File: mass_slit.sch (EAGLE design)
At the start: 31 parts, among them IC1 PIC18F1220P

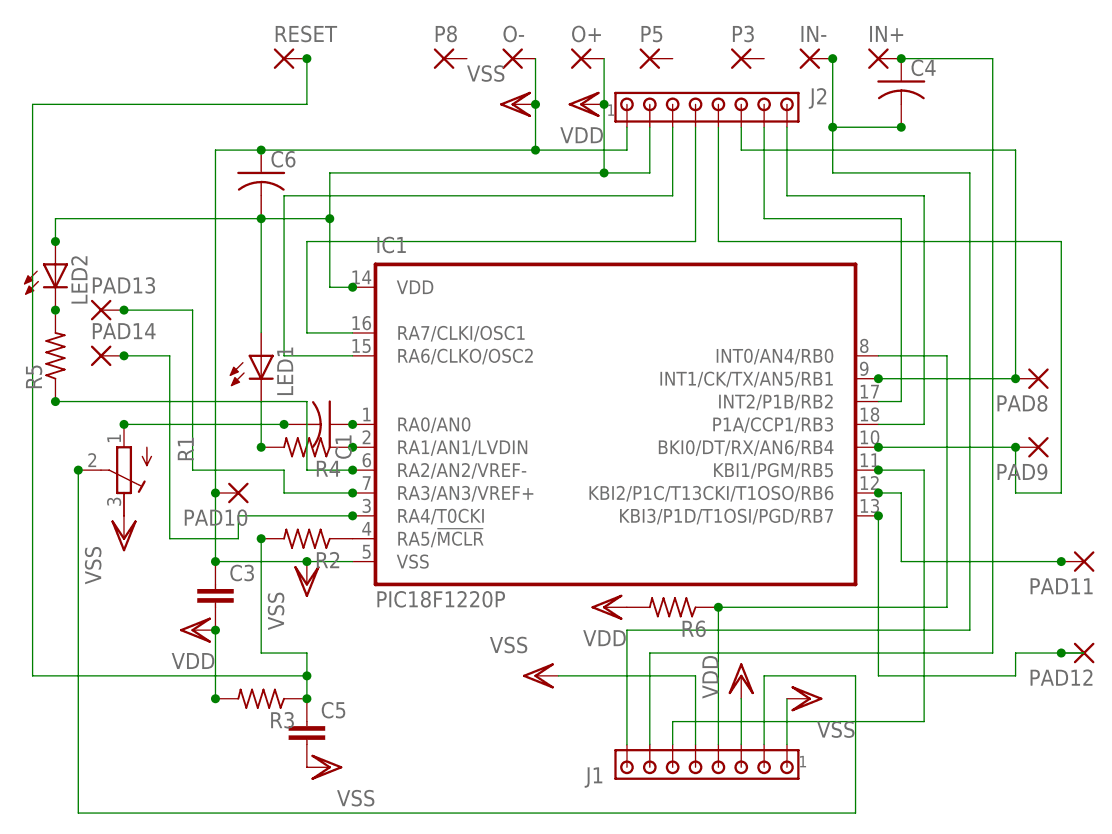
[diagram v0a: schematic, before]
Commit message: up
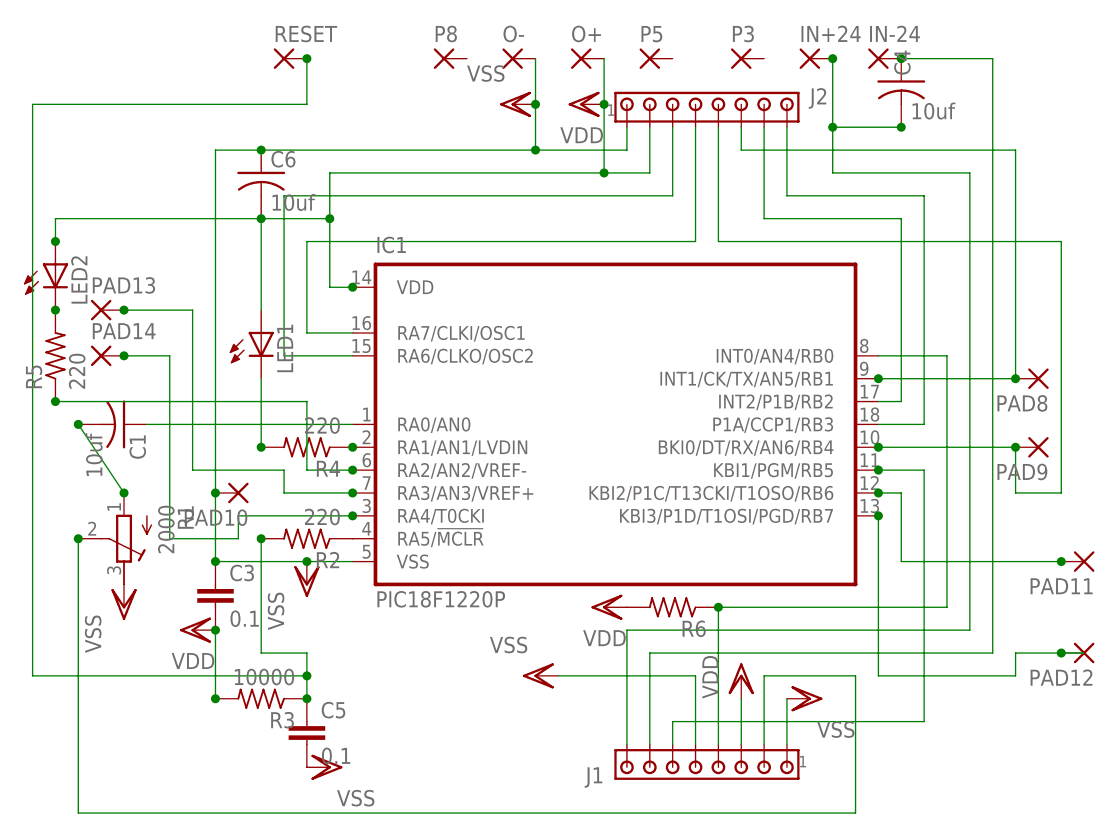
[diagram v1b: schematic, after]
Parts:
- C1, C4, C6: value (none) -> 10uf
- C3, C5: value (none) -> 0.1
- R1: value (none) -> 2000
- R2, R4, R5: value (none) -> 220
- R3: value (none) -> 10000
- renumbered IN+ to IN-24, IN- to IN+24
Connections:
- net N$5 renamed -24
- net N$6 renamed +24
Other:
- moved on the sheet: C1, LED1, R1
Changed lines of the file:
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@@
 <?xml version="1.0" encoding="utf-8"?>
 <!DOCTYPE eagle SYSTEM "eagle.dtd">
-<eagle version="9.2.2">
+<eagle version="9.4.1">
 <drawing>
 <settings>
@@
 <part name="P5" library="wirepad" deviceset="1,6/0,9" device=""/>
 <part name="P3" library="wirepad" deviceset="1,6/0,9" device=""/>
-<part name="IN-" library="wirepad" deviceset="1,6/0,9" device=""/>
-<part name="IN+" library="wirepad" deviceset="1,6/0,9" device=""/>
+<part name="IN+24" library="wirepad" deviceset="1,6/0,9" device=""/>
+<part name="IN-24" library="wirepad" deviceset="1,6/0,9" device=""/>
 <part name="VSS1" library="supply1" deviceset="VSS" device=""/>
-<part name="C1" library="resistor" deviceset="C-US" device="025-040X050"/>
-<part name="C3" library="capacitor-wima" deviceset="C" device="5/2.5"/>
-<part name="C4" library="resistor" deviceset="C-US" device="025-040X050"/>
-<part name="C5" library="capacitor-wima" deviceset="C" device="5/2.5"/>
-<part name="C6" library="resistor" deviceset="C-US" device="025-040X050"/>
+<part name="C1" library="resistor" deviceset="C-US" device="025-040X050" value="10uf"/>
+<part name="C3" library="capacitor-wima" deviceset="C" device="5/2.5" value="0.1"/>
+<part name="C4" library="resistor" deviceset="C-US" device="025-040X050" value="10uf"/>
+<part name="C5" library="capacitor-wima" deviceset="C" device="5/2.5" value="0.1"/>
+<part name="C6" library="resistor" deviceset="C-US" device="025-040X050" value="10uf"/>
 <part name="J1" library="con-amp" deviceset="MTA08-100" device=""/>
-<part name="R1" library="resistor" deviceset="R-TRIMM" device="3339P"/>
-<part name="R2" library="resistor" deviceset="R-US_" device="0204/2V"/>
-<part name="R3" library="resistor" deviceset="R-US_" device="0204/2V"/>
-<part name="R4" library="resistor" deviceset="R-US_" device="0204/2V"/>
+<part name="R1" library="resistor" deviceset="R-TRIMM" device="3339P" value="2000"/>
+<part name="R2" library="resistor" deviceset="R-US_" device="0204/2V" value="220"/>
+<part name="R3" library="resistor" deviceset="R-US_" device="0204/2V" value="10000"/>
+<part name="R4" library="resistor" deviceset="R-US_" device="0204/2V" value="220"/>
 <part name="VSS4" library="supply1" deviceset="VSS" device=""/>
 <part name="VSS5" library="supply1" deviceset="VSS" device=""/>
@@
 <part name="PAD14" library="wirepad" deviceset="1,6/0,9" device=""/>
 <part name="RESET" library="wirepad" deviceset="1,6/0,9" device=""/>
-<part name="R5" library="resistor" deviceset="R-US_" device="0204/2V"/>
+<part name="R5" library="resistor" deviceset="R-US_" device="0204/2V" value="220"/>
 <part name="LED2" library="led" deviceset="LED" device="3MM"/>
 </parts>
@@
 <attribute name="VALUE" x="80.137" y="90.678" size="1.778" layer="96"/>
 </instance>
-<instance part="IN-" gate="1" x="88.9" y="93.98" smashed="yes">
+<instance part="IN+24" gate="1" x="88.9" y="93.98" smashed="yes">
 <attribute name="NAME" x="87.757" y="95.8342" size="1.778" layer="95"/>
 <attribute name="VALUE" x="87.757" y="90.678" size="1.778" layer="96"/>
 </instance>
-<instance part="IN+" gate="1" x="96.52" y="93.98" smashed="yes">
+<instance part="IN-24" gate="1" x="96.52" y="93.98" smashed="yes">
 <attribute name="NAME" x="95.377" y="95.8342" size="1.778" layer="95"/>
 <attribute name="VALUE" x="95.377" y="90.678" size="1.778" layer="96"/>
@@
 <attribute name="VALUE" x="30.48" y="30.48" size="1.778" layer="96" rot="R90"/>
 </instance>
-<instance part="C1" gate="G$1" x="35.56" y="53.34" smashed="yes" rot="R270">
-<attribute name="NAME" x="36.195" y="52.324" size="1.778" layer="95" rot="R270"/>
-<attribute name="VALUE" x="31.369" y="52.324" size="1.778" layer="96" rot="R270"/>
+<instance part="C1" gate="G$1" x="12.7" y="53.34" smashed="yes" rot="R270">
+<attribute name="NAME" x="13.335" y="52.324" size="1.778" layer="95" rot="R270"/>
+<attribute name="VALUE" x="8.509" y="52.324" size="1.778" layer="96" rot="R270"/>
 </instance>
 <instance part="C3" gate="G$1" x="22.86" y="35.56" smashed="yes">
@@
 </instance>
 <instance part="C4" gate="G$1" x="99.06" y="91.44" smashed="yes">
-<attribute name="NAME" x="100.076" y="92.075" size="1.778" layer="95"/>
+<attribute name="NAME" x="100.076" y="92.075" size="1.778" layer="95" rot="R90"/>
 <attribute name="VALUE" x="100.076" y="87.249" size="1.778" layer="96"/>
 </instance>
@@
 <attribute name="VALUE" x="66.04" y="19.05" size="1.778" layer="96" rot="R180"/>
 </instance>
-<instance part="R1" gate="G$1" x="12.7" y="48.26" smashed="yes" rot="R180">
-<attribute name="NAME" x="18.669" y="52.07" size="1.778" layer="95" rot="R270"/>
-<attribute name="VALUE" x="16.51" y="52.07" size="1.778" layer="96" rot="R270"/>
+<instance part="R1" gate="G$1" x="12.7" y="40.64" smashed="yes" rot="R180">
+<attribute name="NAME" x="18.669" y="44.45" size="1.778" layer="95" rot="R270"/>
+<attribute name="VALUE" x="16.51" y="44.45" size="1.778" layer="96" rot="R270"/>
 </instance>
 <instance part="R2" gate="G$1" x="33.02" y="40.64" smashed="yes" rot="R180">
@@
 <attribute name="VALUE" x="36.83" y="54.102" size="1.778" layer="96" rot="R180"/>
 </instance>
-<instance part="VSS4" gate="G$1" x="12.7" y="40.64" smashed="yes">
-<attribute name="VALUE" x="10.16" y="35.56" size="1.778" layer="96" rot="R90"/>
+<instance part="VSS4" gate="G$1" x="12.7" y="33.02" smashed="yes">
+<attribute name="VALUE" x="10.16" y="27.94" size="1.778" layer="96" rot="R90"/>
 </instance>
 <instance part="VSS5" gate="G$1" x="88.9" y="22.86" smashed="yes" rot="R90">
 <attribute name="VALUE" x="93.98" y="20.32" size="1.778" layer="96" rot="R180"/>
 </instance>
-<instance part="LED1" gate="G$1" x="27.94" y="60.96" smashed="yes">
-<attribute name="NAME" x="31.496" y="56.388" size="1.778" layer="95" rot="R90"/>
-<attribute name="VALUE" x="33.655" y="56.388" size="1.778" layer="96" rot="R90"/>
+<instance part="LED1" gate="G$1" x="27.94" y="63.5" smashed="yes">
+<attribute name="NAME" x="31.496" y="58.928" size="1.778" layer="95" rot="R90"/>
+<attribute name="VALUE" x="33.655" y="58.928" size="1.778" layer="96" rot="R90"/>
 </instance>
 <instance part="PAD8" gate="1" x="114.3" y="58.42" smashed="yes" rot="R180">
@@
 <junction x="66.04" y="88.9"/>
 <pinref part="LED1" gate="G$1" pin="A"/>
-<wire x1="27.94" y1="76.2" x2="27.94" y2="63.5" width="0.1524" layer="91"/>
+<wire x1="27.94" y1="76.2" x2="27.94" y2="66.04" width="0.1524" layer="91"/>
 <wire x1="27.94" y1="76.2" x2="5.08" y2="76.2" width="0.1524" layer="91"/>
 <pinref part="LED2" gate="G$1" pin="A"/>
@@
 <pinref part="IC1" gate="G$1" pin="RA0/AN0"/>
 <pinref part="C1" gate="G$1" pin="1"/>
-<junction x="38.1" y="53.34"/>
+<wire x1="15.24" y1="53.34" x2="38.1" y2="53.34" width="0.1524" layer="91"/>
 </segment>
 </net>
@@
 <segment>
 <pinref part="C1" gate="G$1" pin="2"/>
-<wire x1="12.7" y1="53.34" x2="30.48" y2="53.34" width="0.1524" layer="91"/>
-<junction x="30.48" y="53.34"/>
+<wire x1="12.7" y1="45.72" x2="7.62" y2="53.34" width="0.1524" layer="91"/>
+<junction x="7.62" y="53.34"/>
 <pinref part="R1" gate="G$1" pin="A"/>
-<junction x="12.7" y="53.34"/>
-</segment>
-</net>
-<net name="N$5" class="0">
-<segment>
-<pinref part="IN+" gate="1" pin="P"/>
+<junction x="12.7" y="45.72"/>
+</segment>
+</net>
+<net name="-24" class="0">
+<segment>
+<pinref part="IN-24" gate="1" pin="P"/>
 <pinref part="C4" gate="G$1" pin="1"/>
 <junction x="99.06" y="93.98"/>
@@
 </segment>
 </net>
-<net name="N$6" class="0">
-<segment>
-<pinref part="IN-" gate="1" pin="P"/>
+<net name="+24" class="0">
+<segment>
+<pinref part="IN+24" gate="1" pin="P"/>
 <wire x1="91.44" y1="93.98" x2="91.44" y2="86.36" width="0.1524" layer="91"/>
 <pinref part="C4" gate="G$1" pin="2"/>
@@
 <segment>
 <pinref part="R1" gate="G$1" pin="S"/>
-<wire x1="7.62" y1="48.26" x2="7.62" y2="10.16" width="0.1524" layer="91"/>
+<wire x1="7.62" y1="40.64" x2="7.62" y2="10.16" width="0.1524" layer="91"/>
 <wire x1="7.62" y1="10.16" x2="93.98" y2="10.16" width="0.1524" layer="91"/>
 <wire x1="93.98" y1="10.16" x2="93.98" y2="25.4" width="0.1524" layer="91"/>
@@
 <pinref part="J1" gate="G$1" pin="2"/>
 <wire x1="83.82" y1="25.4" x2="83.82" y2="17.78" width="0.1524" layer="91"/>
-<junction x="7.62" y="48.26"/>
+<junction x="7.62" y="40.64"/>
 </segment>
 </net>
@@
 <pinref part="LED1" gate="G$1" pin="C"/>
 <pinref part="R4" gate="G$1" pin="2"/>
-<wire x1="27.94" y1="55.88" x2="27.94" y2="50.8" width="0.1524" layer="91"/>
+<wire x1="27.94" y1="58.42" x2="27.94" y2="50.8" width="0.1524" layer="91"/>
 <junction x="27.94" y="50.8"/>
 </segment>
